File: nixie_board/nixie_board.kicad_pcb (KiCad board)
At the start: 2 copper layers, 227.3 x 61 mm, 68 parts, among them J1 12V, J2 170V, J3 GND, J4 SHDN, J5 Barrel_Jack_Switch, Q1 MPSA42, Q2 MPSA42, U1 74LS32, U10 74LS32, U11 K155ID1, U12 L7805, U13 74HCT595, U14 K155ID1, U15 DS18B20, U2 K155ID1, U3 WeMos_D1_mini, U4 74HCT595, U5 K155ID1, U6 74LS32, U7 K155ID1, U8 74HCT595, U9 K155ID1

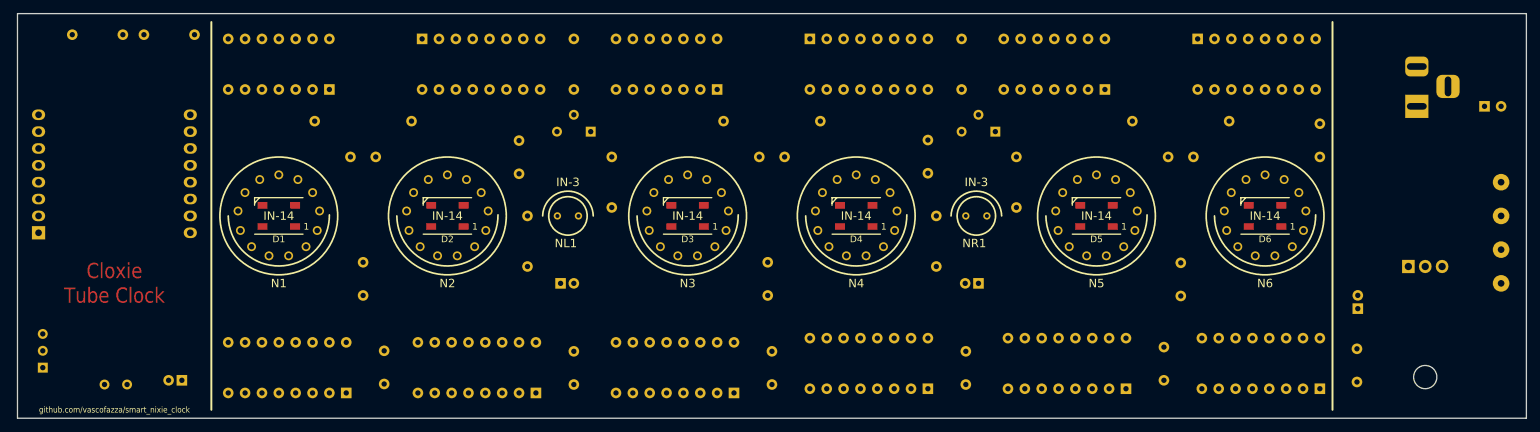
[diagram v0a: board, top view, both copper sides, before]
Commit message: pcb REV1
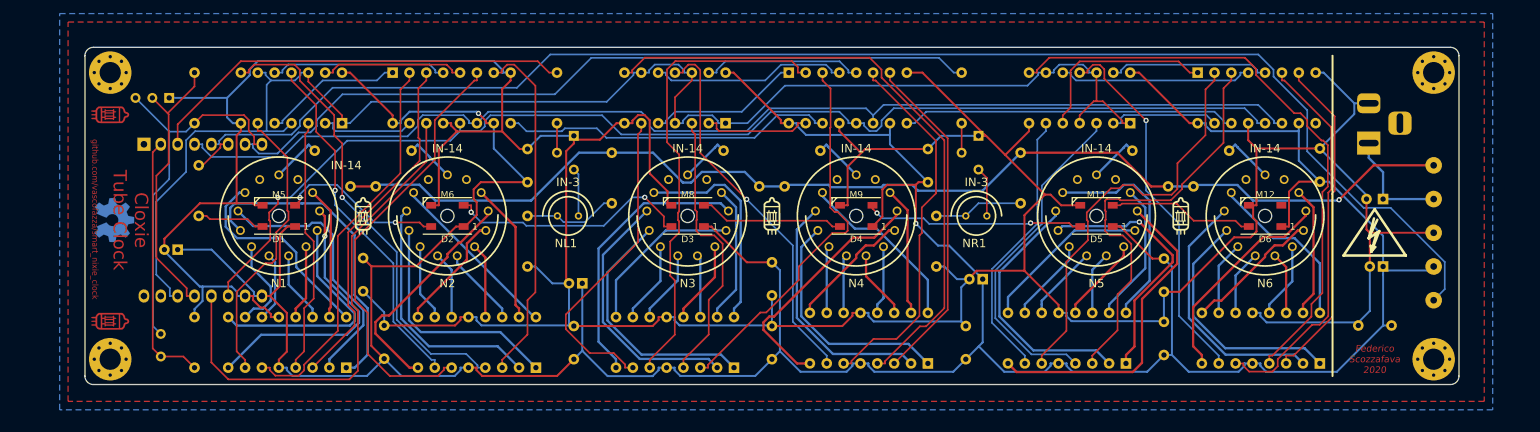
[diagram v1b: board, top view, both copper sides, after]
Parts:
- removed U12: L7805, Package_TO_SOT_THT:TO-220-3_Horizontal_TabDown
- added J6: 5V, Connector_Wire:SolderWirePad_1x01_Drill1mm, B.Cu at (254.0, 59.7)
- added M1: MountingHole_3.2mm_M3_Pad_Via, MountingHole:MountingHole_3.2mm_M3_Pad_Via, F.Cu at (254.0, 30.5)
- added M11: MountingHole_2mm, MountingHole:MountingHole_2mm, F.Cu at (203.2, 52.1)
- added M12: MountingHole_2mm, MountingHole:MountingHole_2mm, F.Cu at (228.6, 52.1)
- added M2: MountingHole_3.2mm_M3_Pad_Via, MountingHole:MountingHole_3.2mm_M3_Pad_Via, F.Cu at (254.0, 73.7)
- added M3: MountingHole_3.2mm_M3_Pad_Via, MountingHole:MountingHole_3.2mm_M3_Pad_Via, F.Cu at (54.6, 73.7)
- added M4: MountingHole_3.2mm_M3_Pad_Via, MountingHole:MountingHole_3.2mm_M3_Pad_Via, F.Cu at (54.6, 30.5)
- added M5: MountingHole_2mm, MountingHole:MountingHole_2mm, F.Cu at (80.0, 52.1)
- added M6: MountingHole_2mm, MountingHole:MountingHole_2mm, F.Cu at (105.4, 52.1)
- added M8: MountingHole_2mm, MountingHole:MountingHole_2mm, F.Cu at (141.6, 52.1)
- added M9: MountingHole_2mm, MountingHole:MountingHole_2mm, F.Cu at (167.0, 52.1)
- added R16: 10K, Resistor_THT:R_Axial_DIN0207_L6.3mm_D2.5mm_P7.62mm_Horizontal, B.Cu at (67.3, 74.9)
- added S0: Symbol_HighVoltage_Type2_CopperTop_VerySmall, Symbol:Symbol_HighVoltage_Type2_CopperTop_VerySmall, F.Cu at (245.1, 55.2)
- added S1: Symbol_Barrel_Polarity, Symbol:Symbol_Barrel_Polarity, B.Cu at (252.1, 38.1)
- added S10: LOGO, Symbol:tube_silk, B.Cu at (154.3, 52.1)
- added S11: LOGO, Symbol:tube_silk, B.Cu at (215.9, 52.1)
- added S12: LOGO, Symbol:tube_silk, F.Cu at (54.6, 36.8)
- added S13: LOGO, Symbol:tube_silk, F.Cu at (54.6, 67.9)
- added S2, S2b: OSHW-Symbol_6.7x6mm_Copper, Symbol:OSHW-Symbol_6.7x6mm_Copper, B.Cu at (55.2, 52.7)
- added S4: LOGO, Symbol:tube, F.Cu at (54.6, 36.8)
- added S5: LOGO, Symbol:tube, F.Cu at (54.6, 67.9)
- added S6: LOGO, Symbol:tube_silk, F.Cu at (154.3, 52.1)
- added S7: LOGO, Symbol:tube_silk, F.Cu at (92.7, 52.1)
- added S8: LOGO, Symbol:tube_silk, F.Cu at (215.9, 52.1)
- added S9: LOGO, Symbol:tube_silk, B.Cu at (92.7, 52.1)
- R10, R14: value 150K -> 130K
- moved U15 44.9 mm to (63.5, 34.3), turned to 180 degrees
- moved R9 22.7 mm to (67.3, 38.1), turned to 90 degrees
- moved R8 21.3 mm to (67.9, 44.5), turned to 270 degrees
- moved U3 20.7 mm to (59.7, 41.3), turned to 270 degrees
- moved C7 20.7 mm to (246.4, 49.5), turned to 180 degrees
- moved J2 20.5 mm to (254.0, 44.5)
- moved C16 19.7 mm to (64.8, 57.1)
- moved J4 12.7 mm to (254.0, 64.8)
- moved J1 10.5 mm to (254.0, 49.5)
- moved J3 10.5 mm to (254.0, 54.6)
- moved R7 9.16 mm to (62.2, 69.8), turned to 270 degrees
- moved J5 9.12 mm to (244.2, 41.1)
- moved C17 7.41 mm to (246.4, 59.7), turned to 180 degrees
- moved U4 6.75 mm to (97.2, 30.5)
- moved U10 6.35 mm to (208.3, 38.1)
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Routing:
- net GND: track 0.00 -> 594.7 mm
- net /5V: track 0.00 -> 552.4 mm, vias 0 -> 2
- net /STROBE: track 0.00 -> 222.4 mm
- net /SHUTDOWN: track 0.00 -> 215.9 mm
- net /RCLK: track 0.00 -> 180.9 mm, vias 0 -> 1
- net /170V: track 0.00 -> 179.2 mm, vias 0 -> 1
- net /SRCLK: track 0.00 -> 176.3 mm
- net /RIGHT_DOT: track 0.00 -> 116.3 mm
- net Net-(U6-Pad8): track 0.00 -> 94.2 mm
- net Net-(U10-Pad8): track 0.00 -> 89.5 mm
- net /SER: track 0.00 -> 76.0 mm
- net Net-(U7-Pad6): track 0.00 -> 70.8 mm
- net Net-(U1-Pad8): track 0.00 -> 70.2 mm, vias 0 -> 1
- net Net-(U4-Pad6): track 0.00 -> 65.7 mm
- net /LEFT_DOT: track 0.00 -> 64.8 mm
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- added copper zone on B.Cu, net GND
- added copper zone on F.Cu, net GND
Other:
- board size 227.3 x 61 mm -> 207 x 50.8 mm
- net class HighVoltageIN: clearance 0.35 -> 0.3; trace_width 0.5 -> 0.35
- net class HighVoltageOut: trace_width 0.4 -> 0.35
- board text added: "+"
- board text added: "-"
- board text added: "12V DC"
- board text added: "Federico Scozzafava 2020"
- board text added: "REV1"
